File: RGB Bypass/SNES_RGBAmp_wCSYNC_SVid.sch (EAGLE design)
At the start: 25 parts, among them U1 THS7374

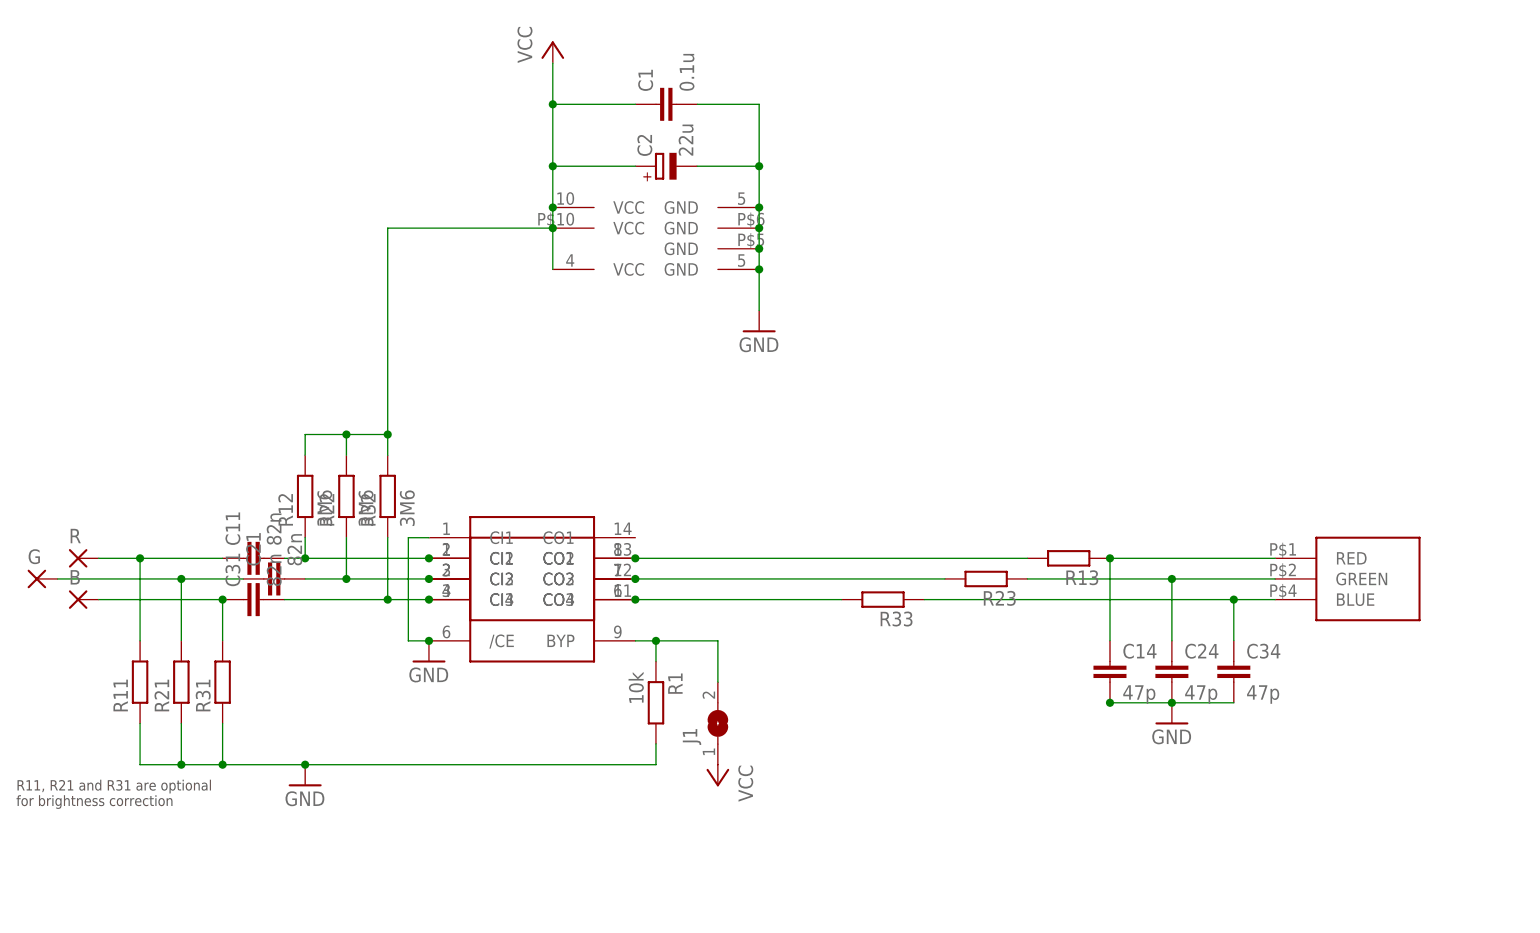
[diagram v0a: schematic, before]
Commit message: go to version 4.1
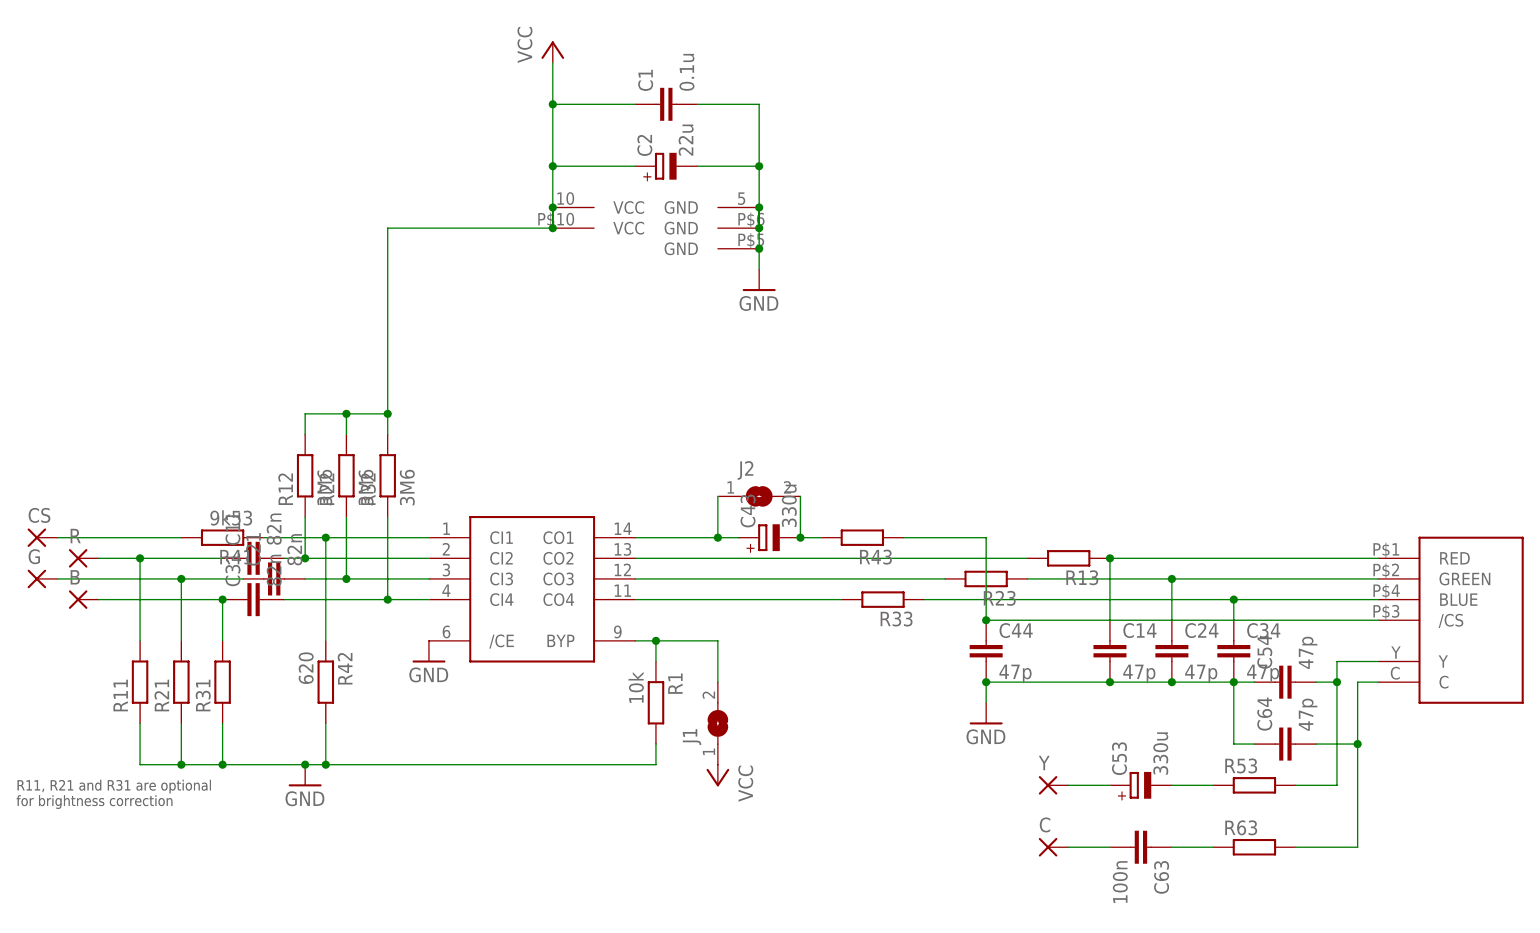
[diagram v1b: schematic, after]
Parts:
- removed U$2: THS7314, snes_div:THS7314
- added C, CS, Y: (no value), wirepad:SMD2
- added C43, C53: 330u, rcl:CPOL-EUSMCD
- added C44, C54, C64: 47p, rcl:C-EUC0603K
- added C63: 100n, rcl:C-EUC0603K
- added J2: (no value), jumper:SJ
- added R41: 9k53, rcl:R-EU_R0603
- added R42: 620, rcl:R-EU_R0603
- added R43, R53, R63: (no value), rcl:R-EU_R0603
- U$1: value SNES_MULTIAV_RGB_ONLY -> SNES_MULTIAV_RGBSYC; device snes_div:SNES_MULTIAV_RGB_ONLY -> snes_div:SNES_MULTIAV_RGBSYC
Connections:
- new net N$10: R41.1, R42.1, U1G$1.CI1
- new net N$11: R33.2, U1G$1.CO4
- new net N$12: C53.+, Y.P
- new net N$13: C.P, C63.2
- new net N$17: CS.P, R41.2
- new net N$18: C43.+, J2.1, U1G$1.CO1
- new net N$19: C43.-, J2.2, R43.2
- new net N$20: C53.-, R53.1
- new net N$21: C54.2, R53.2, U$1G$1.Y
- new net N$22: C64.2, R63.2, U$1G$1.C
- new net N$23: C63.1, R63.1
- net GND: now also C44.2, C54.1, C64.1, R42.2, U$1G$3.GND; no longer U$1G$1.GND, U$2G$2.GND, U1G$1.CI1
- net N$1: no longer U$2G$1.CI1
- net N$2: no longer U$2G$1.CI2
- net N$4: now also C44.1, R43.1, U$1G$1./CS; no longer R23.2, U$2G$1.CO2, U1G$1.CO3
- net N$5: now also U$1G$1.RED; no longer U$1G$3.RED
- net N$6: now also U$1G$1.GREEN; no longer U$1G$3.GREEN
- net N$7: now also R23.2, U1G$1.CO3; no longer R13.2, U$2G$1.CO1, U1G$1.CO2
- net N$8: now also R13.2, U1G$1.CO2; no longer R33.2, U$2G$1.CO3, U1G$1.CO4
- net N$9: now also U$1G$1.BLUE; no longer U$1G$3.BLUE
- net R9: no longer U$2G$1.CI3
- net VCC: now also U$1G$3.VCC; no longer U$1G$2.VCC, U$2G$2.VCC
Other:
- moved on the sheet: C14, C24, C34, R12, R22, R32
